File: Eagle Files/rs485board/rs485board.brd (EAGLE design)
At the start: 63.2 x 63.5 mm, 59 parts, among them IC1 XC6206P332MR, IC2 MP2359, J1 AVR_SPI_PROG_3X2PTH, J2 RA 6Pin SMD, Q1 CJ3404, Q2 CJ3404, Q3 CJ3404, U1 ATMEGA328P_TQFP, U2 LIS3DH, U3 MAX3485CSA, X1 RJ45-8L-B, X2 RJ45-8L-B, Y1 16MHz

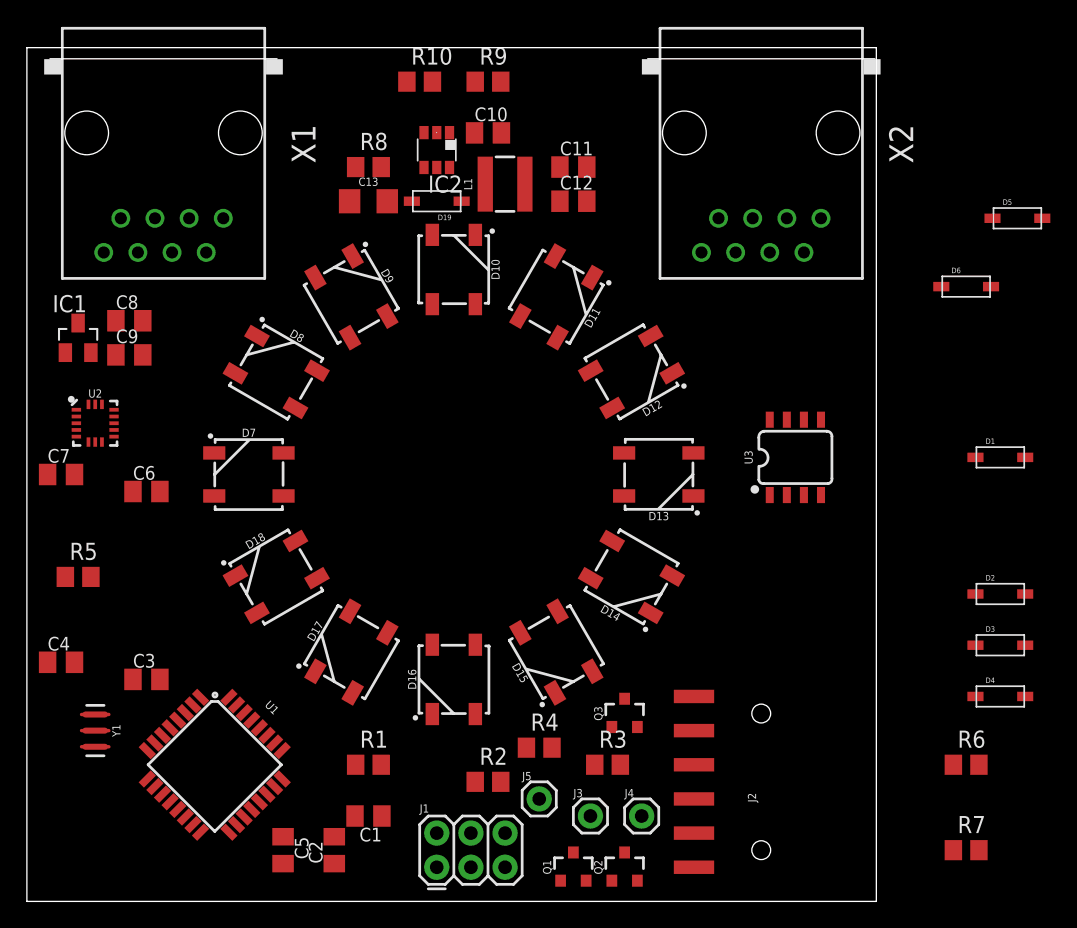
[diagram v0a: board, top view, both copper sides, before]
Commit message: add more traces
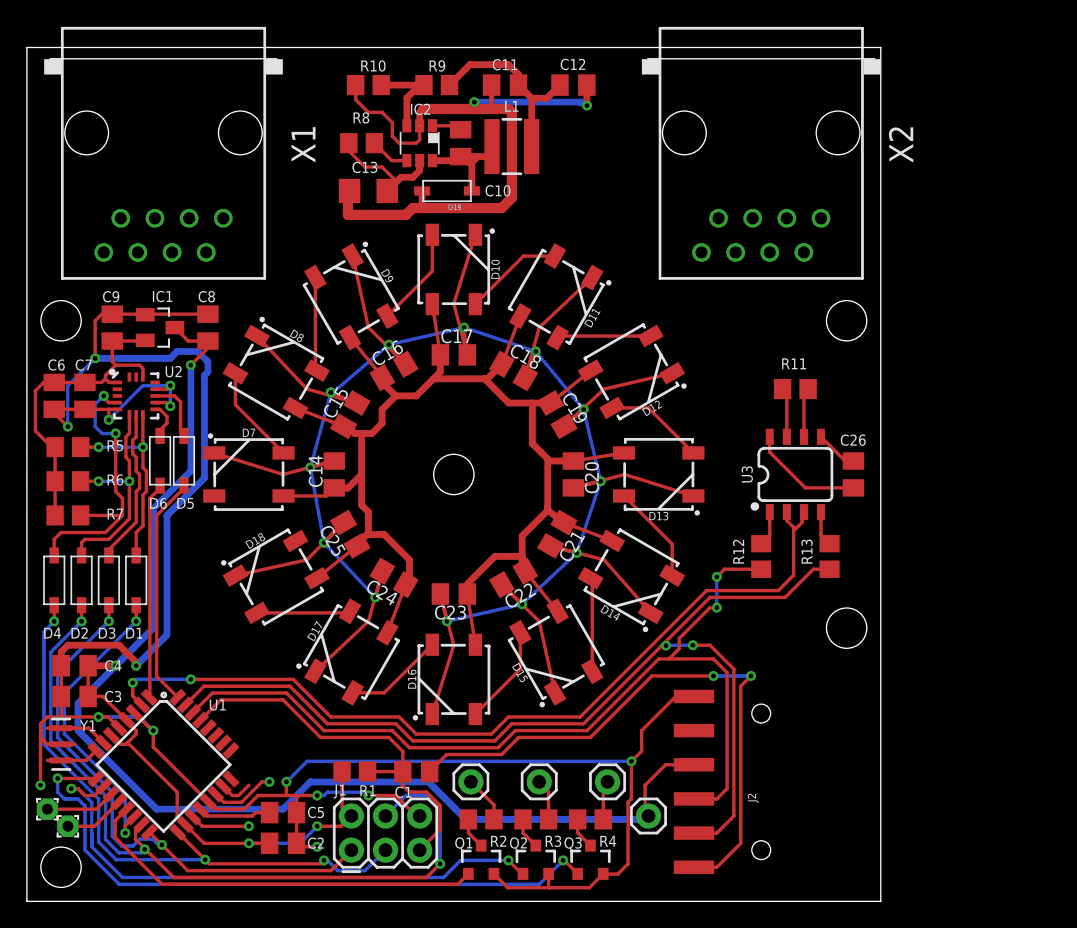
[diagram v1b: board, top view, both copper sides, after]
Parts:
- added C14, C15, C16, C17, C18, C19, C20, C21, C22, C23, C24, C25, C26: (no value), resistor:C0805K
- added J6: (no value), SparkFun-Connectors:1X01
- added PAD1, PAD2: (no value), wirepad:1,6/0,8
- added R11, R12, R13: (no value), resistor:R0805
- moved R7 71.3 mm to (3.05, 28.7), turned to 180 degrees
- moved D4 70.9 mm to (2.03, 23.9), turned to 90 degrees
- moved R6 70.0 mm to (3.05, 31.2), turned to 180 degrees
- moved D2 68.3 mm to (4.06, 23.9), turned to 90 degrees
- moved D3 66.5 mm to (6.10, 23.9), turned to 90 degrees
- moved D1 64.9 mm to (8.13, 23.9), turned to 90 degrees
- moved D5 64.5 mm to (11.7, 32.8), turned to 90 degrees
- moved D6 61.3 mm to (9.91, 32.8), turned to 90 degrees
- moved Q3 11.2 mm to (41.9, 3.05)
- moved C6 9.88 mm to (2.03, 37.6), turned to 270 degrees
- moved R5 9.68 mm to (3.05, 33.8), turned to 180 degrees
- moved J3 9.25 mm to (33.0, 8.89)
- moved C12 8.64 mm to (40.6, 60.7)
- moved J4 8.03 mm to (38.1, 8.89)
- moved C11 7.94 mm to (35.6, 60.7), turned to 180 degrees
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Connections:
- new net +5V6: C14.1, D7.1
- new net A0: U1.23
- new net A1: U1.24
- new net A2: U1.25
- new net A3: U1.26
- new net A4: U1.27
- new net A5: U1.28
- new net A6: U1.19
- new net A7: U1.22
- new net D7: PAD1.1, U1.11
- new net D8: PAD2.1, U1.12
- new net DIR: U1.2, U3.2, U3.3
- new net N$20: R11.2, U3.7, X1.1, X2.1
- new net N$22: R11.1, U3.6, X1.2, X2.2
- new net N$30: R12.2, U3.1
- new net N$31: R13.2, U3.4
- net +24V: now also X1.4, X1.5, X2.4, X2.5
- net +3V3: no longer C2.1, C3.1, C4.1, U1.18, U1.4, U1.6
- net +5V: now also C15.1, C16.1, C17.1, C18.1, C19.1, C2.1, C20.1, C21.1, C22.1, C23.1, C24.1, C25.1, C26.1, C3.1, C4.1, D10.1, D11.1, D12.1, D13.1, D14.1, D15.1, D16.1, D17.1, D18.1, D8.1, D9.1, J6.1, U1.18, U1.4, U1.6, U3.8
- net GND: now also C14.2, C15.2, C16.2, C17.2, C18.2, C19.2, C20.2, C21.2, C22.2, C23.2, C24.2, C25.2, C26.2, D10.3, D11.3, D12.3, D13.3, D14.3, D15.3, D16.3, D17.3, D18.3, D7.3, D8.3, D9.3, U3.5, X1.3, X1.6, X1.7, X1.8, X2.3, X2.6, X2.7, X2.8
- net RX: now also R12.1
- net TX: now also R13.1
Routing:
- net GND: track 0.00 -> 434.4 mm, vias 0 -> 29
- net +5V: track 0.00 -> 257.8 mm, vias 0 -> 4
- net TX: track 0.00 -> 75.9 mm, vias 0 -> 2
- net RX: track 0.00 -> 68.0 mm, vias 0 -> 2
- net DIR: track 0.00 -> 64.4 mm, vias 0 -> 2
- net MOSI: track 0.00 -> 58.4 mm, vias 0 -> 3
- net D5: track 0.00 -> 48.5 mm, vias 0 -> 2
- net SCK: track 0.00 -> 45.6 mm, vias 0 -> 3
- net RESET_EXT: track 0.00 -> 44.1 mm, vias 0 -> 2
- net D6: track 0.00 -> 43.1 mm, vias 0 -> 2
- net MISO: track 0.00 -> 41.7 mm, vias 0 -> 2
- net D9: track 0.00 -> 30.5 mm
- net RESET: track 0.00 -> 29.8 mm
- net +3V3: track 0.00 -> 25.4 mm
- net SS: track 0.00 -> 22.6 mm, vias 0 -> 2
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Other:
- board size 63.2 x 63.5 mm -> 63.5 x 63.5 mm
